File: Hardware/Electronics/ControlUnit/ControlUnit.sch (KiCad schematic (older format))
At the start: 78 parts, among them J1 Screw_Terminal_01x02, Batt 9V, J10 S3, J11 MPU-6050/MPU-9250, J12 S4, J13 Conn_01x02, J2 USB_B_Mini, J3 Conn_01x05, J4 Conn_Coaxial, J5 Conn_Coaxial, J6 Micro_SD_Card, J7 S1, J8 BME280, J9 S2, Q1 , Q2 , SW1 SW_DPDT_x2, SW2 SW_Push, U1 ATSAMD21G18A-AFT, U2 LM340_SOT223/LM7805_5V, U3 MCP1826S_3.3V, U4 RFM69W, U5 MAX-8Q, U6 W25Q32JVSS, Y1 32.768kHz

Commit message: Encore
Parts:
- C22: footprint (none) -> Capacitor_SMD:C_0805_2012Metric
- D1: footprint (none) -> Diode_THT:D_DO-41_SOD81_P10.16mm_Horizontal
- R16: footprint (none) -> Resistor_SMD:R_0805_2012Metric
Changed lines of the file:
@@
 Wire Wire Line
 	3500 2500 3500 1650
-Wire Wire Line
-	3800 2500 3800 2400
 NoConn ~ 10850 5700
 Wire Notes Line
@@
 State indicators
 $Comp
-L Device:D_Zener D1
-U 1 1 608DBB45
-P 2550 8150
-F 0 "D1" V 2504 8230 50  0000 L CNN
-F 1 "D_Zener" V 2595 8230 50  0000 L CNN
-F 2 "" H 2550 8150 50  0001 C CNN
-F 3 "~" H 2550 8150 50  0001 C CNN
-	1    2550 8150
-	0    1    1    0
-$EndComp
-$Comp
 L Transistor_FET:BS250 Q2
 U 1 1 6091F04D
@@
 F 0 "R16" H 2320 8546 50  0000 L CNN
 F 1 "10k" H 2320 8455 50  0000 L CNN
-F 2 "" V 2180 8500 50  0001 C CNN
+F 2 "Resistor_SMD:R_0805_2012Metric" V 2180 8500 50  0001 C CNN
 F 3 "~" H 2250 8500 50  0001 C CNN
 	1    2250 8500
@@
 F 0 "C22" H 4800 9750 50  0000 L CNN
 F 1 "100n" H 4800 9650 50  0000 L CNN
-F 2 "" H 5138 9550 50  0001 C CNN
+F 2 "Capacitor_SMD:C_0805_2012Metric" H 5138 9550 50  0001 C CNN
 F 3 "~" H 5100 9700 50  0001 C CNN
 	1    5100 9700
@@
 	1    0    0    -1
 $EndComp
+Wire Wire Line
+	3800 2500 3800 2400
+$Comp
+L Device:D_Zener D1
+U 1 1 608DBB45
+P 2550 8150
+F 0 "D1" V 2504 8230 50  0000 L CNN
+F 1 "D_Zener" V 2595 8230 50  0000 L CNN
+F 2 "Diode_THT:D_DO-41_SOD81_P10.16mm_Horizontal" H 2550 8150 50  0001 C CNN
+F 3 "~" H 2550 8150 50  0001 C CNN
+	1    2550 8150
+	0    1    1    0
+$EndComp
 $EndSCHEMATC

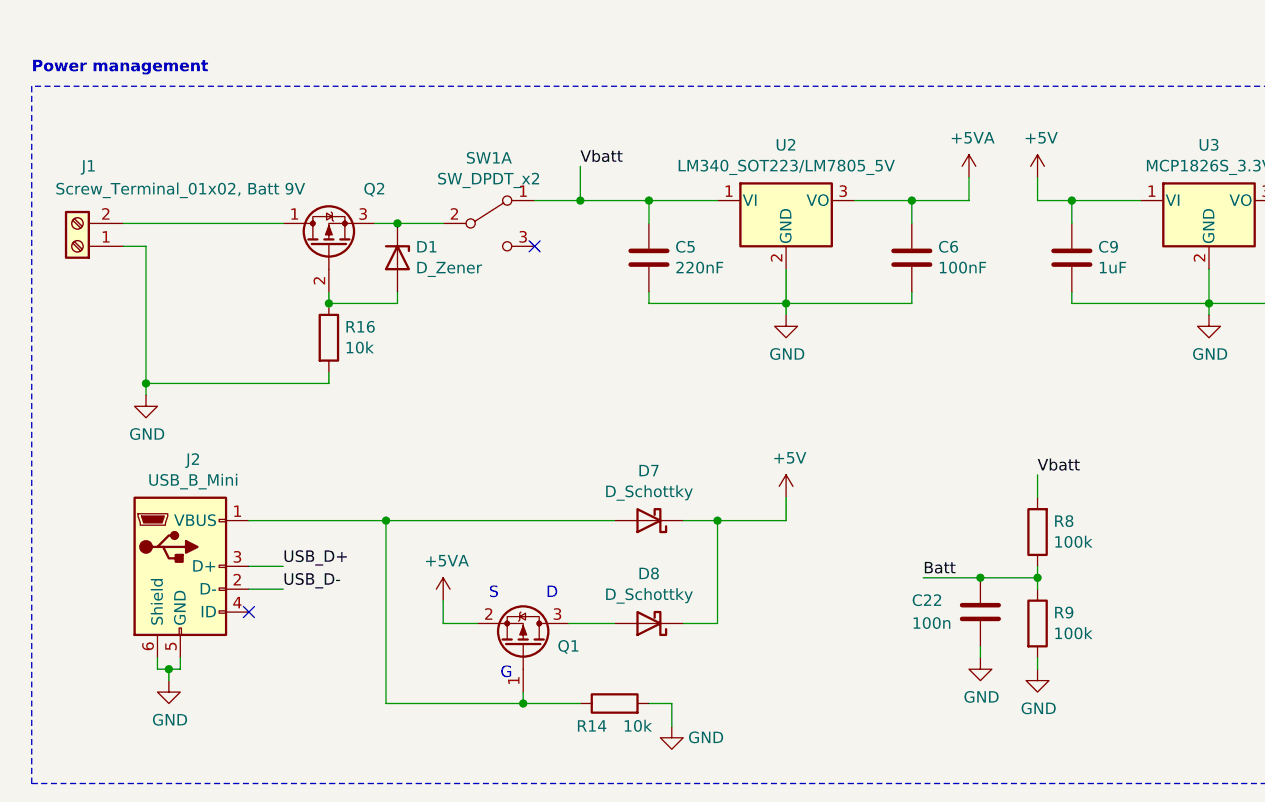
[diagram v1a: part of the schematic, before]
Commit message: Encore
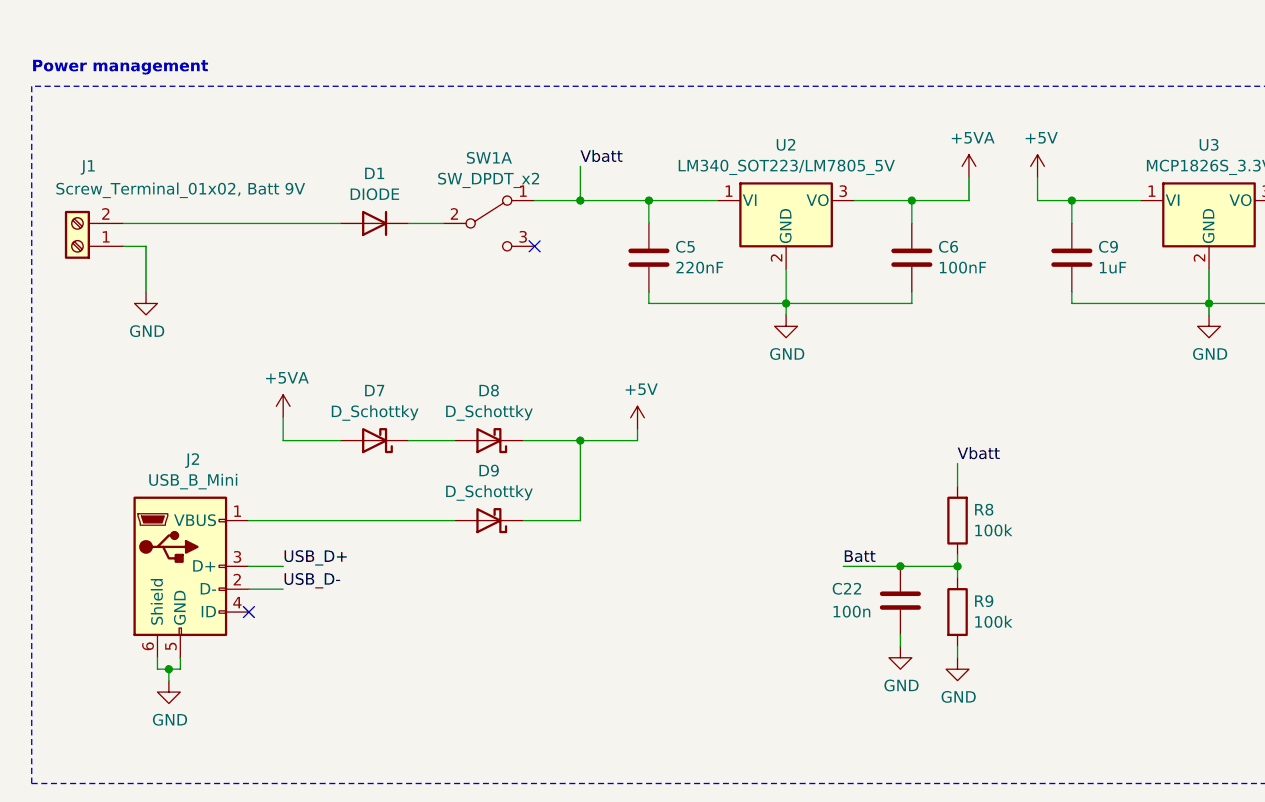
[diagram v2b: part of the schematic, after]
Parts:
- removed D1: D_Zener, Diode_THT:D_DO-41_SOD81_P10.16mm_Horizontal, symbol Device:D_Zener
- removed Q1: (no value), Package_TO_SOT_SMD:SOT-23, symbol Transistor_FET:AO3401A
- removed Q2: (no value), Package_TO_SOT_SMD:SOT-23, symbol Transistor_FET:BS250
- removed R14, R16: 10k, Resistor_SMD:R_0805_2012Metric, symbol Device:R
- added D1: DIODE, Diode_THT:D_DO-41_SOD81_P10.16mm_Horizontal, symbol Simulation_SPICE:DIODE
- added D9: D_Schottky, CustomLib:DIOM5436X244N, symbol Device:D_Schottky
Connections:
- net +5V: now also D9.1 (K); no longer D7.1 (K)
- net +5VA: now also D7.2 (A)
- net at SW1.2 (B): now also D1.2 (K)
- net at J2.1 (VBUS): now also D9.2 (A); no longer D7.2 (A)
- net at D8.2 (A): now also D7.1 (K)
- net at J1.2 (Pin_2): now also D1.1 (A)
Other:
- note removed: "D"
- note removed: "G"
- note removed: "S"
- moved on the sheet: C22, D7, D8, R8, R9
